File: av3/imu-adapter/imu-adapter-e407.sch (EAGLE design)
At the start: 20 parts, among them J1 CLM-112-02, J2 TSM-116-DV

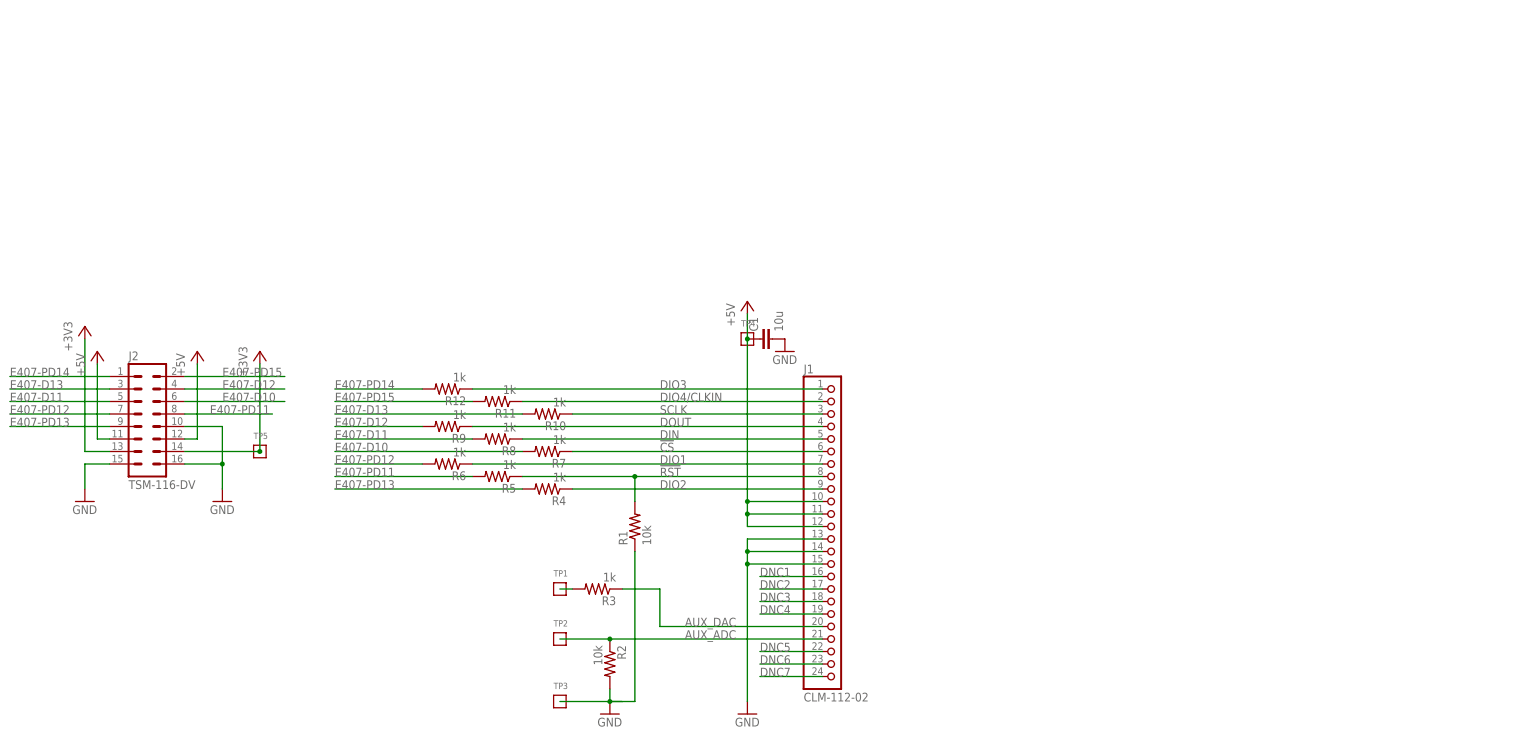
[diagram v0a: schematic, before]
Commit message: Added stupid EAGLE temporary files to the gitignore. Updated IMU adapter with sane net names so we could easily trace nets. And updated the e407 shield to add a RGB LED, correct some schematic mistakes found out while double checking connections, and updated to being routable on a PCB router.
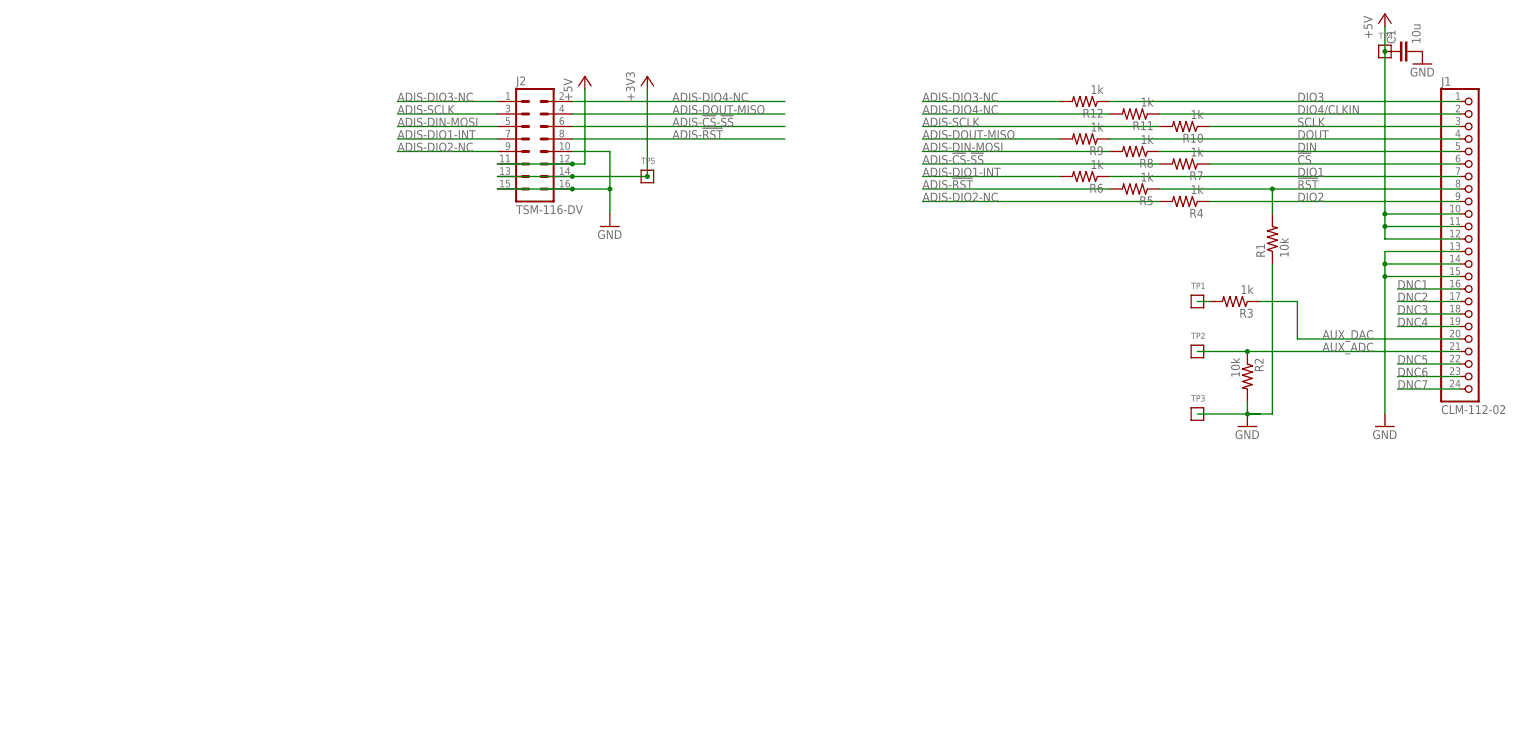
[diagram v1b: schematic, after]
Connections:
- net E407-D10 renamed ADIS-!CS!-!SS
- net E407-D11 renamed ADIS-DIN-MOSI
- net E407-D12 renamed ADIS-DOUT-MISO
- net E407-D13 renamed ADIS-SCLK
- net E407-PD11 renamed ADIS-!RST
- net E407-PD12 renamed ADIS-DIO1-INT
- net E407-PD13 renamed ADIS-DIO2-NC
- net E407-PD14 renamed ADIS-DIO3-NC
- net E407-PD15 renamed ADIS-DIO4-NC
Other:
- moved on the sheet: C1, J1, J2, R1, R10, R11, R12, R2, R3, R4, R5, R6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
